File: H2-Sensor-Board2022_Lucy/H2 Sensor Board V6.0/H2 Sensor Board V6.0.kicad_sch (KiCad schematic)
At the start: 1 part, among them U1 STM32L442KCUx

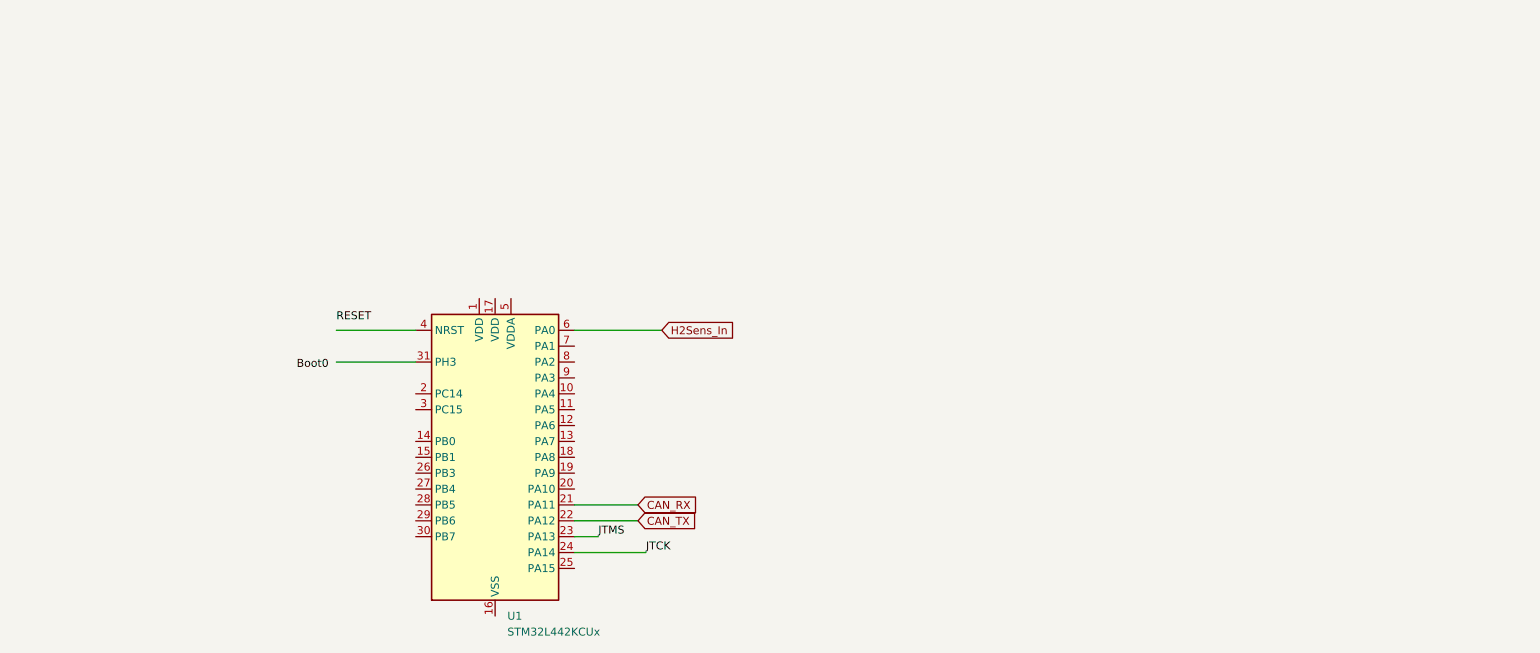
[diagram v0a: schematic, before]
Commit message: W
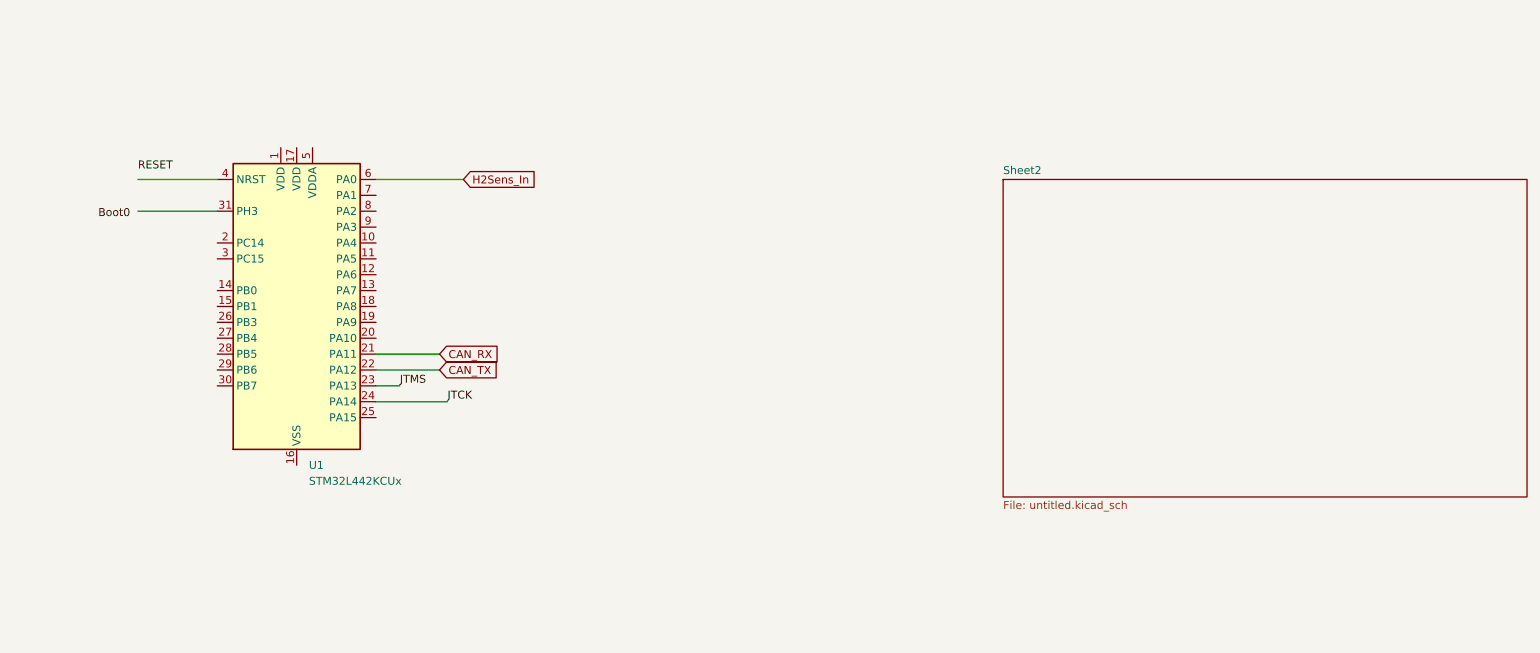
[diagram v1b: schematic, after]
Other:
- added sheet Sheet2 (untitled.kicad_sch)
- moved on the sheet: U1
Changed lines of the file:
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@@
 (kicad_sch (version 20230121) (generator eeschema)
   (paper "A4")
-  (wire (pts (xy 109.22 100.33) (xy 113.03 100.33))
+  (wire (pts (xy 77.47 76.2) (xy 81.28 76.2))
     (stroke (width 0) (type default))
   )
-  (wire (pts (xy 109.22 95.25) (xy 119.38 95.25))
+  (wire (pts (xy 77.47 71.12) (xy 87.63 71.12))
     (stroke (width 0) (type default))
   )
-  (wire (pts (xy 109.22 102.87) (xy 120.65 102.87))
+  (wire (pts (xy 77.47 78.74) (xy 88.9 78.74))
     (stroke (width 0) (type default))
   )
-  (wire (pts (xy 71.12 67.31) (xy 83.82 67.31))
+  (wire (pts (xy 39.37 43.18) (xy 52.07 43.18))
     (stroke (width 0) (type default))
   )
-  (wire (pts (xy 109.22 97.79) (xy 119.38 97.79))
+  (wire (pts (xy 77.47 73.66) (xy 87.63 73.66))
     (stroke (width 0) (type default))
   )
-  (wire (pts (xy 71.12 72.39) (xy 83.82 72.39))
+  (wire (pts (xy 39.37 48.26) (xy 52.07 48.26))
     (stroke (width 0) (type default))
   )
-  (wire (pts (xy 109.22 67.31) (xy 123.19 67.31))
+  (wire (pts (xy 77.47 43.18) (xy 91.44 43.18))
     (stroke (width 0) (type default))
   )
-  (label "JTCK" (at 120.65 102.87 0) (fields_autoplaced)
+  (label "JTCK" (at 88.9 78.74 0) (fields_autoplaced)
     (effects (font (size 1.27 1.27)) (justify left bottom))
   )
-  (label "JTMS" (at 113.03 100.33 0) (fields_autoplaced)
+  (label "JTMS" (at 81.28 76.2 0) (fields_autoplaced)
     (effects (font (size 1.27 1.27)) (justify left bottom))
   )
-  (label "RESET" (at 71.12 66.04 0) (fields_autoplaced)
+  (label "RESET" (at 39.37 41.91 0) (fields_autoplaced)
     (effects (font (size 1.27 1.27)) (justify left bottom))
   )
-  (label "Boot0" (at 64.77 73.66 0) (fields_autoplaced)
+  (label "Boot0" (at 33.02 49.53 0) (fields_autoplaced)
     (effects (font (size 1.27 1.27)) (justify left bottom))
   )
-  (global_label "H2Sens_In" (shape input) (at 123.19 67.31 0) (fields_autoplaced)
+  (global_label "H2Sens_In" (shape input) (at 91.44 43.18 0) (fields_autoplaced)
     (effects (font (size 1.27 1.27)) (justify left))
-    (property "Intersheetrefs" "${INTERSHEET_REFS}" (at 135.9118 67.31 0)
+    (property "Intersheetrefs" "${INTERSHEET_REFS}" (at 104.1618 43.18 0)
       (effects (font (size 1.27 1.27)) (justify left) hide)
     )
   )
-  (global_label "CAN_RX" (shape input) (at 119.38 95.25 0) (fields_autoplaced)
+  (global_label "CAN_RX" (shape input) (at 87.63 71.12 0) (fields_autoplaced)
     (effects (font (size 1.27 1.27)) (justify left))
-    (property "Intersheetrefs" "${INTERSHEET_REFS}" (at 129.5014 95.25 0)
+    (property "Intersheetrefs" "${INTERSHEET_REFS}" (at 97.7514 71.12 0)
       (effects (font (size 1.27 1.27)) (justify left) hide)
     )
   )
-  (global_label "CAN_TX" (shape input) (at 119.38 97.79 0) (fields_autoplaced)
+  (global_label "CAN_TX" (shape input) (at 87.63 73.66 0) (fields_autoplaced)
     (effects (font (size 1.27 1.27)) (justify left))
-    (property "Intersheetrefs" "${INTERSHEET_REFS}" (at 129.199 97.79 0)
+    (property "Intersheetrefs" "${INTERSHEET_REFS}" (at 97.449 73.66 0)
       (effects (font (size 1.27 1.27)) (justify left) hide)
     )
   )
-  (symbol (lib_id "MCU_ST_STM32L4:STM32L442KCUx") (at 96.52 87.63 0) (unit 1)
+  (symbol (lib_id "MCU_ST_STM32L4:STM32L442KCUx") (at 64.77 63.5 0) (unit 1)
     (in_bom yes) (on_board yes) (dnp no) (fields_autoplaced)
-    (property "Reference" "U1" (at 98.4759 113.03 0)
+    (property "Reference" "U1" (at 66.7259 88.9 0)
       (effects (font (size 1.27 1.27)) (justify left))
     )
-    (property "Value" "STM32L442KCUx" (at 98.4759 115.57 0)
+    (property "Value" "STM32L442KCUx" (at 66.7259 91.44 0)
       (effects (font (size 1.27 1.27)) (justify left))
     )
-    (property "Footprint" "Package_DFN_QFN:QFN-32-1EP_5x5mm_P0.5mm_EP3.45x3.45mm" (at 86.36 110.49 0)
+    (property "Footprint" "Package_DFN_QFN:QFN-32-1EP_5x5mm_P0.5mm_EP3.45x3.45mm" (at 54.61 86.36 0)
       (effects (font (size 1.27 1.27)) (justify right) hide)
     )
-    (property "Datasheet" "https://www.st.com/resource/en/datasheet/stm32l442kc.pdf" (at 96.52 87.63 0)
+    (property "Datasheet" "https://www.st.com/resource/en/datasheet/stm32l442kc.pdf" (at 64.77 63.5 0)
       (effects (font (size 1.27 1.27)) hide)
     )
@@
       )
     )
+  )
+  (sheet (at 177.8 43.18) (size 83.82 50.8) (fields_autoplaced)
+    (stroke (width 0.1524) (type solid))
+    (fill (color 0 0 0 0.0000))
+    (property "Sheetname" "Sheet2" (at 177.8 42.4684 0)
+      (effects (font (size 1.27 1.27)) (justify left bottom))
+    )
+    (property "Sheetfile" "untitled.kicad_sch" (at 177.8 94.5646 0)
+      (effects (font (size 1.27 1.27)) (justify left top))
+    )
+    (instances
+      (project "H2 Sensor Board V6.0"
+        (path "/61fdd4a1-2d1e-44dc-8644-252e12d35745" (page "2"))
+      )
+    )

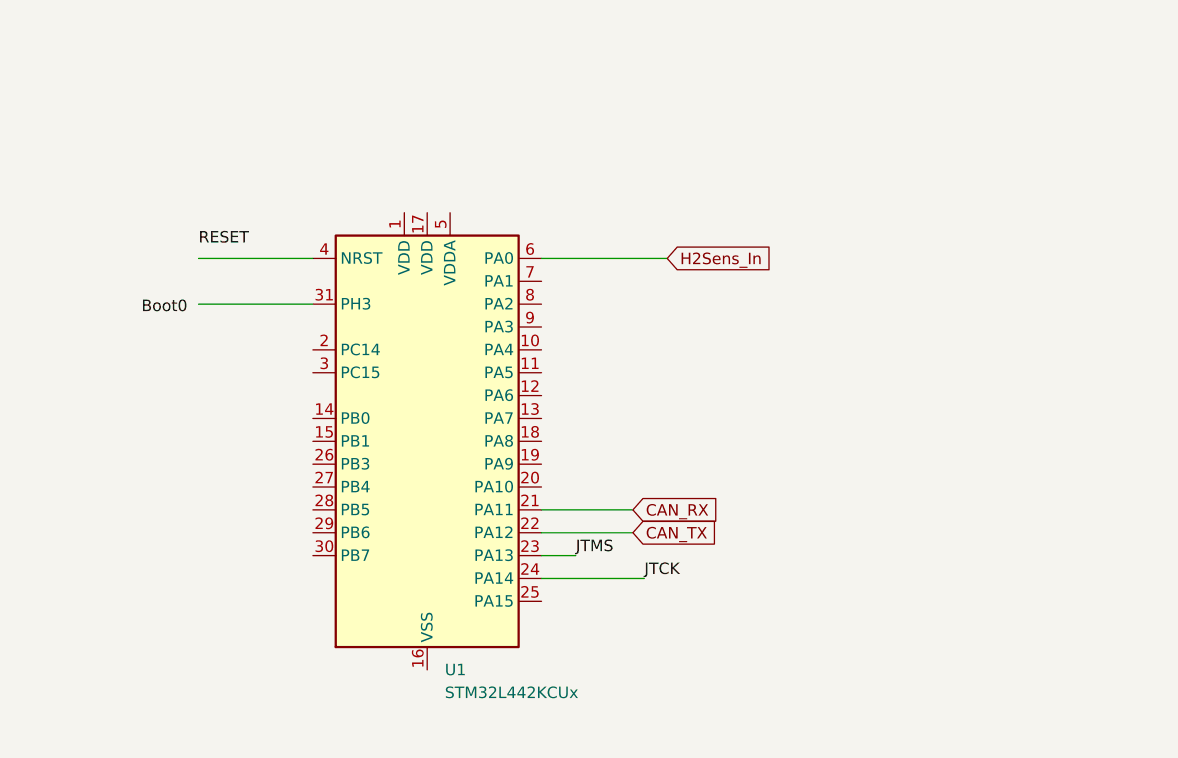
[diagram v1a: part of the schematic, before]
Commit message: up
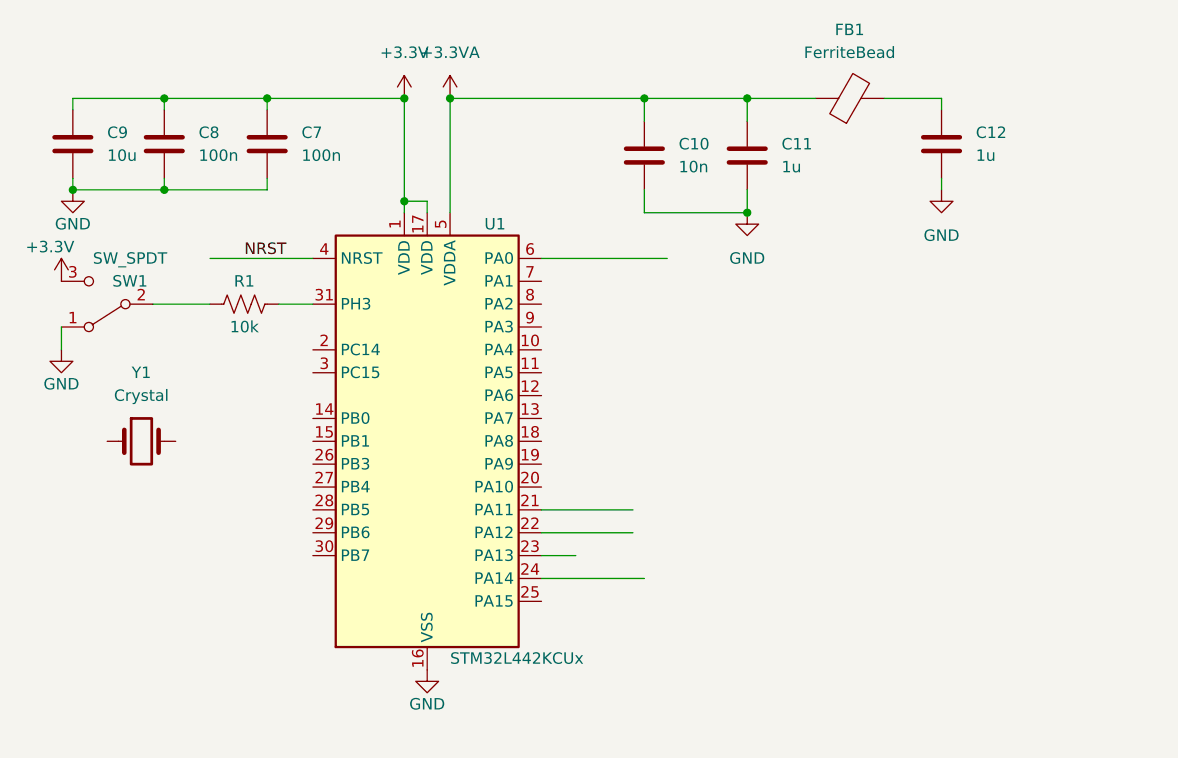
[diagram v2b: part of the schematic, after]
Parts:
- added C10: 10n, symbol Device:C
- added C11, C12: 1u, symbol Device:C
- added C7, C8: 100n, symbol Device:C
- added C9: 10u, symbol Device:C
- added FB1: FerriteBead, symbol Device:FerriteBead
- added R1: 10k, symbol Device:R_US
- added SW1: SW_SPDT, symbol Switch:SW_SPDT
- added Y1: Crystal, symbol Device:Crystal
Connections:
- net +3.3V: now reaches U1.1 (VDD)
- net +3.3V: now also U1.17 (VDD), C7.1, C8.1, C9.1, SW1.3 (C)
- net GND: now reaches U1.16 (VSS), U1.32 (VSS), U1.33 (VSS)
- net GND: now also C10.2, C11.2, C12.2, C7.2, C8.2, C9.2, SW1.1 (A)
- net at U1.31 (PH3): now also R1.2
- net NRST: now reaches U1.4 (NRST)
- net +3.3VA: now reaches U1.5 (VDDA)
- net +3.3VA: now also C10.1, C11.1, FB1.1
- net CAN_RX: no longer names the net of U1.21 (PA11)
- net CAN_TX: no longer names the net of U1.22 (PA12)
- net H2Sens_In: no longer names the net of U1.6 (PA0)
- net JTCK: no longer names the net of U1.24 (PA14)
- net JTMS: no longer names the net of U1.23 (PA13)
- new net: C12.1, FB1.2
- new net: R1.1, SW1.2 (B)
